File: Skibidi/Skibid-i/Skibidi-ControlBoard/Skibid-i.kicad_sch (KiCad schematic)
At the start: 53 parts, among them IC1 TEENSY_4.1, J10 Screw_Terminal_01x03, J12 Screw_Terminal_01x03, J13 P78E05-1000, J15 Conn_01x03_Pin, J17 Conn_01x08_Pin, J19 12V, J2 Screw_Terminal_01x03, J20 Screw_Terminal_01x03, J21 Motor1, J22 Motor2, J3 Screw_Terminal_01x03, J4 Screw_Terminal_01x03, J5 Screw_Terminal_01x03, J6 Screw_Terminal_01x03, J7 Screw_Terminal_01x03, J8 Screw_Terminal_01x03, J9 Screw_Terminal_01x03, Q1 WL-OCPT_SERIES_357, Q2 WL-OCPT_SERIES_357, Q3 WL-OCPT_SERIES_357, Q4 WL-OCPT_SERIES_357, Q5 WL-OCPT_SERIES_357, Q6 WL-OCPT_SERIES_357, Q7 WL-OCPT_SERIES_357, SW2 210-4MS

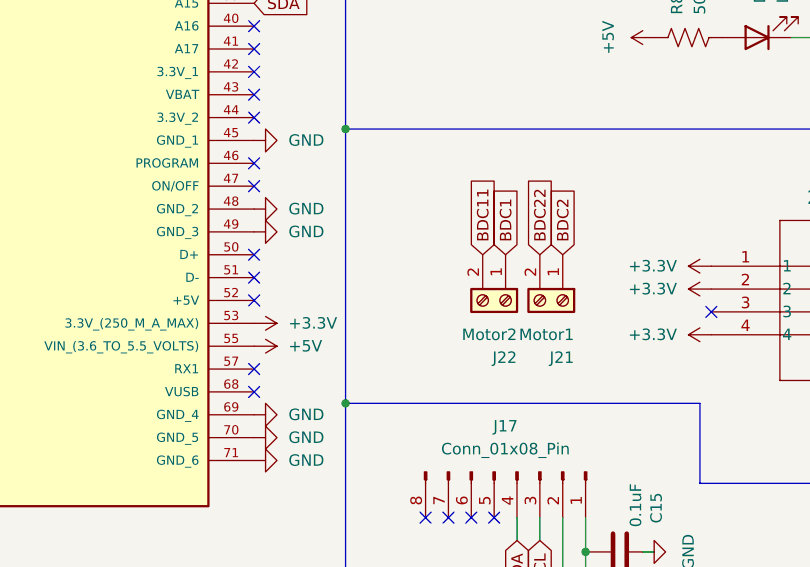
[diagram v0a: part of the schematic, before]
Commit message: sigma fanum
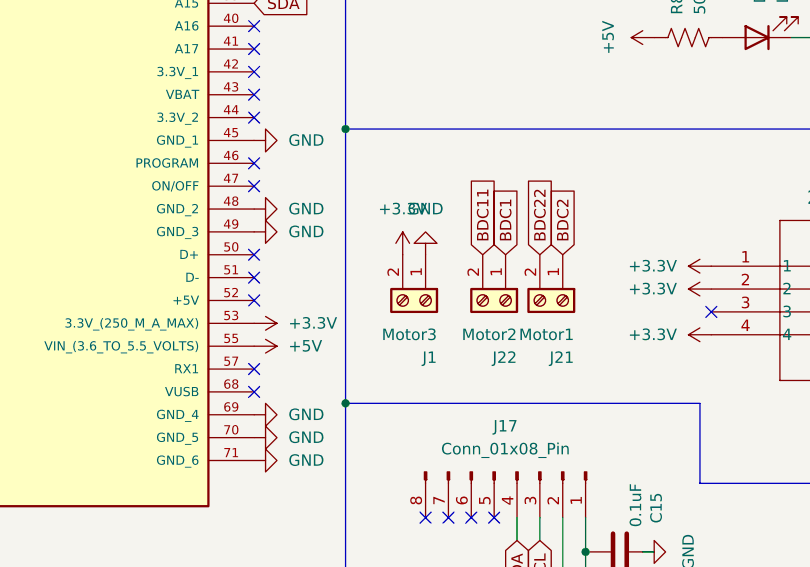
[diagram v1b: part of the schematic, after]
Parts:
- added J1: Motor3, askibidi:Screwterminal2, symbol Connector:Screw_Terminal_01x02
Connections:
- net +3.3V: now also J1.2 (Pin_2)
- net GND: now also J1.1 (Pin_1)
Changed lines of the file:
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@@
 	)
 	(symbol
+		(lib_id "Connector:Screw_Terminal_01x02")
+		(at 190.5 92.71 270)
+		(unit 1)
+		(exclude_from_sim no)
+		(in_bom yes)
+		(on_board yes)
+		(dnp no)
+		(property "Reference" "J1"
+			(at 191.77 99.06 90)
+			(effects
+				(font
+					(size 1.27 1.27)
+				)
+				(justify right)
+			)
+		)
+		(property "Value" "Motor3"
+			(at 191.77 96.52 90)
+			(effects
+				(font
+					(size 1.27 1.27)
+				)
+				(justify right)
+			)
+		)
+		(property "Footprint" "askibidi:Screwterminal2"
+			(at 190.5 92.71 0)
+			(effects
+				(font
+					(size 1.27 1.27)
+				)
+				(hide yes)
+			)
+		)
+		(property "Datasheet" "~"
+			(at 190.5 92.71 0)
+			(effects
+				(font
+					(size 1.27 1.27)
+				)
+				(hide yes)
+			)
+		)
+		(property "Description" ""
+			(at 190.5 92.71 0)
+			(effects
+				(font
+					(size 1.27 1.27)
+				)
+				(hide yes)
+			)
+		)
+		(pin "1"
+		)
+		(pin "2"
+		)
+		(instances
+			(project "Skibid-i"
+				(path "/bfc511a5-2c92-46fd-9868-0fe25107d7eb"
+					(reference "J1")
+					(unit 1)
+				)
+			)
+		)
+	)
+	(symbol
 		(lib_id "Connector:Screw_Terminal_01x03")
 		(at 57.15 48.26 180)
@@
 	)
 	(symbol
+		(lib_name "+3.3V_1")
+		(lib_id "power:+3.3V")
+		(at 187.96 87.63 0)
+		(unit 1)
+		(exclude_from_sim no)
+		(in_bom yes)
+		(on_board yes)
+		(dnp no)
+		(fields_autoplaced yes)
+		(property "Reference" "#PWR059"
+			(at 187.96 91.44 0)
+			(effects
+				(font
+					(size 1.27 1.27)
+				)
+				(hide yes)
+			)
+		)
+		(property "Value" "+3.3V"
+			(at 187.96 82.55 0)
+			(effects
+				(font
+					(size 1.27 1.27)
+				)
+			)
+		)
+		(property "Footprint" ""
+			(at 187.96 87.63 0)
+			(effects
+				(font
+					(size 1.27 1.27)
+				)
+				(hide yes)
+			)
+		)
+		(property "Datasheet" ""
+			(at 187.96 87.63 0)
+			(effects
+				(font
+					(size 1.27 1.27)
+				)
+				(hide yes)
+			)
+		)
+		(property "Description" "Power symbol creates a global label with name \"+3.3V\""
+			(at 187.96 87.63 0)
+			(effects
+				(font
+					(size 1.27 1.27)
+				)
+				(hide yes)
+			)
+		)
+		(pin "1"
+		)
+		(instances
+			(project ""
+				(path "/bfc511a5-2c92-46fd-9868-0fe25107d7eb"
+					(reference "#PWR059")
+					(unit 1)
+				)
+			)
+		)
+	)
+	(symbol
 		(lib_id "Device:C")
 		(at 63.5 30.48 0)
@@
 					(unit 1)
 				)
+			)
+		)
+	)
+	(symbol
+		(lib_name "GND_2")
+		(lib_id "power:GND")
+		(at 190.5 87.63 180)
+		(unit 1)
+		(exclude_from_sim no)
+		(in_bom yes)
+		(on_board yes)
+		(dnp no)
+		(fields_autoplaced yes)
+		(property "Reference" "#PWR061"
+			(at 190.5 81.28 0)
+			(effects
+				(font
+					(size 1.27 1.27)
+				)
+				(hide yes)
+			)
+		)
+		(property "Value" "GND"
+			(at 190.5 82.55 0)
+			(effects
+				(font
+					(size 1.27 1.27)
+				)
+			)
+		)
+		(property "Footprint" ""
+			(at 190.5 87.63 0)
+			(effects
+				(font
+					(size 1.27 1.27)
+				)
+				(hide yes)
+			)
+		)
+		(property "Datasheet" ""
+			(at 190.5 87.63 0)
+			(effects
+				(font
+					(size 1.27 1.27)
+				)
+				(hide yes)
+			)
+		)
+		(property "Description" "Power symbol creates a global label with name \"GND\" , ground"
+			(at 190.5 87.63 0)
+			(effects
+				(font
+					(size 1.27 1.27)
+				)
+				(hide yes)
+			)
+		)
+		(pin "1"
+		)
+		(instances
+			(project ""
+				(path "/bfc511a5-2c92-46fd-9868-0fe25107d7eb"
+					(reference "#PWR061")
+					(unit 1)
+				)

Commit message: done with contrl board
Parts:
- C2: footprint askibidi:Ecap -> Capacitor_SMD:C_2220_5750Metric
- D1: footprint askibidi:LED -> LED_SMD:LED_1206_3216Metric
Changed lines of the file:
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@@
 			)
 		)
-		(property "Footprint" "askibidi:Ecap"
+		(property "Footprint" "Capacitor_SMD:C_2220_5750Metric"
 			(at 246.6848 34.29 0)
 			(effects
@@
 			)
 		)
-		(property "Footprint" "askibidi:LED"
+		(property "Footprint" "LED_SMD:LED_1206_3216Metric"
 			(at 227.33 63.5 0)
 			(effects
